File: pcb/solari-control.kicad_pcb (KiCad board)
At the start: 2 copper layers, 80 x 90 mm, 111 parts, among them J1 Conn_01x04, J2 A5081WV-5P, J3 A5081WR-5P, J4 AVR-ISP-6, J5 DIL8, J6 Conn_01x04, Q1 AO3401A, Q10 BC847, Q11 BC857, Q12 BC847, Q2 2N7002, Q3 BC857, Q4 2N7002, Q5 BSS83, Q6 BSS83, Q7 AO3401A, Q8 AO3401A, Q9 BC857, U1 VO0631T, U10 PC817, U11 PC817, U13 ADuM1201AR, U2 L78L05_SOT89, U3 VO0631T, U4 PC817, U5 PC817, U6 VO0631T, U7 ATmega328P-A, U8 VO0631T, U9 VO0631T, Y1 14.7456 MHz

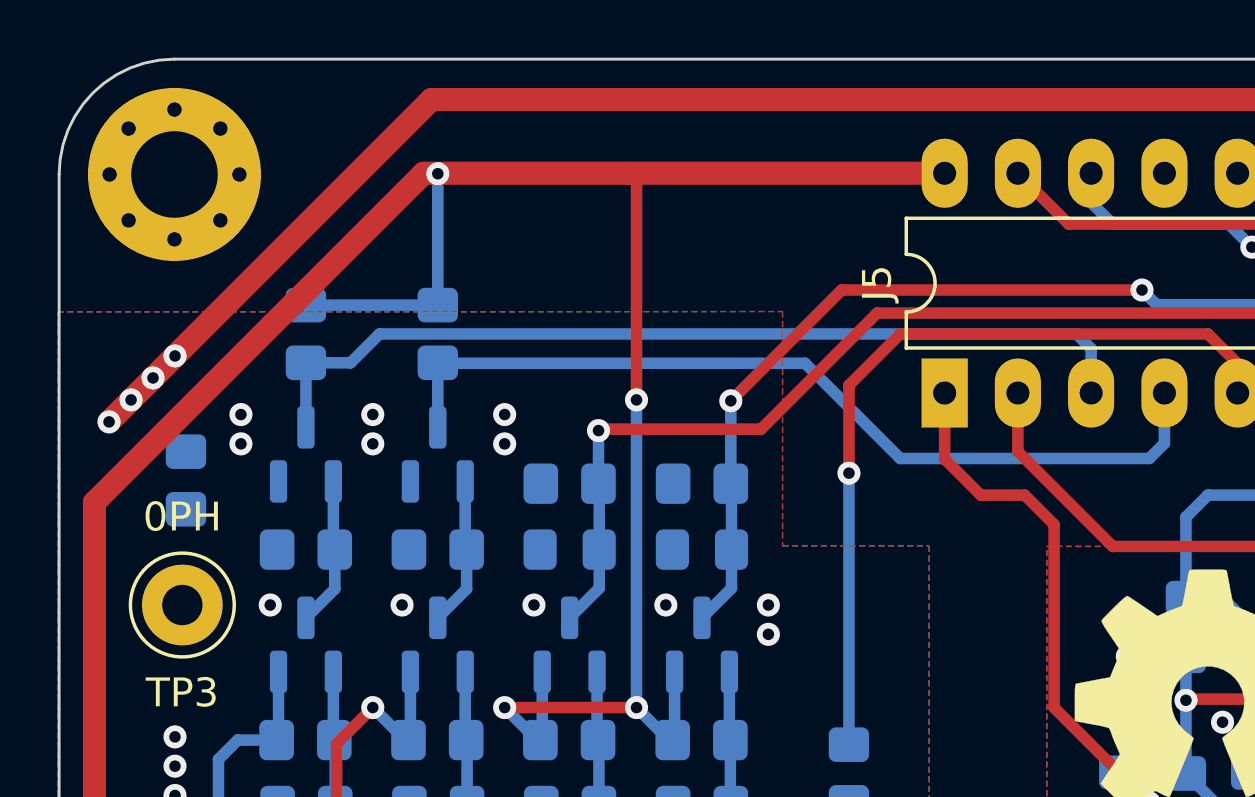
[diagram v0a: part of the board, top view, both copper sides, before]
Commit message: Place new resistor on PCB.
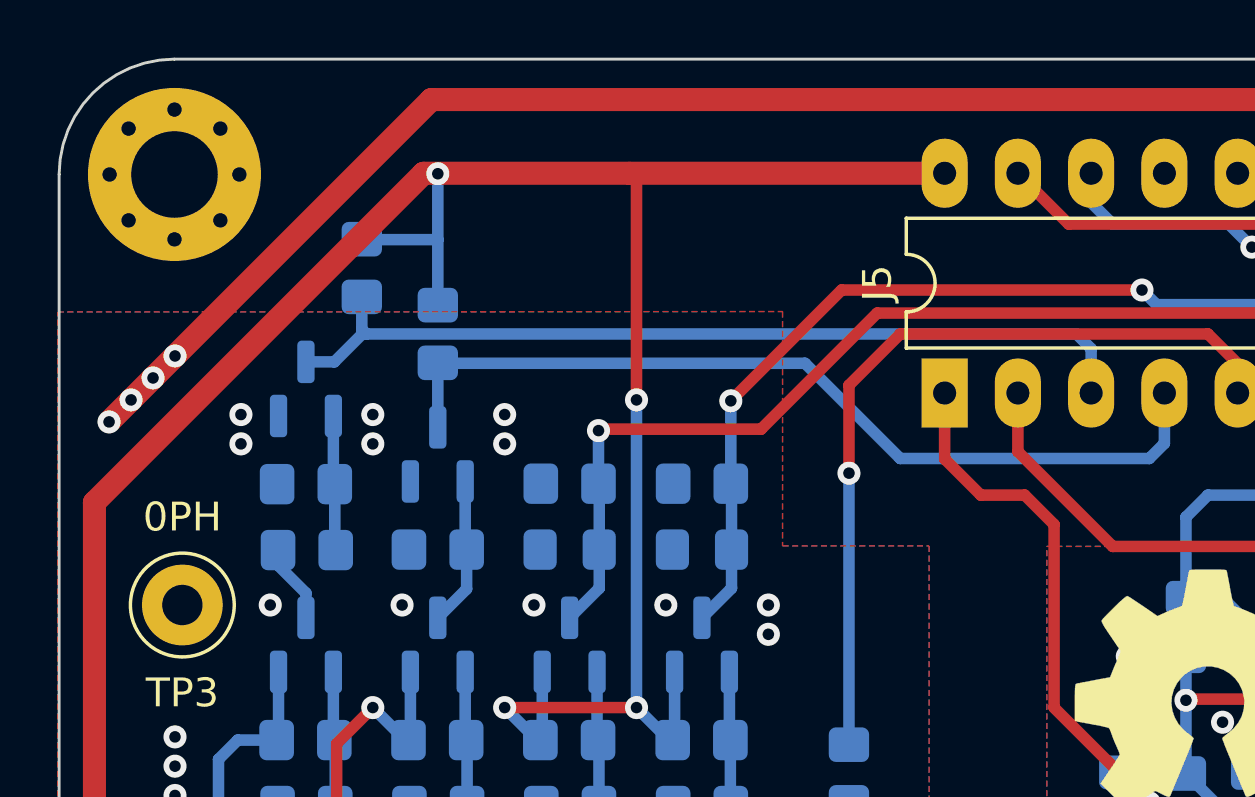
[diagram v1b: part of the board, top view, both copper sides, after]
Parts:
- moved R39 4.84 mm to (148.6, 57.0), turned to 180 degrees
- moved R7 3.00 mm to (150.5, 47.2)
- moved Q4 2.27 mm to (148.6, 51.4)
- moved R12 2.27 mm to (148.6, 54.7)
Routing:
- net Net-(Q3-Pad3): track 0.00 -> 2.75 mm
- net VPH: track 139.3 -> 137.3 mm
- net /CLOCKS: track 31.6 -> 30.7 mm
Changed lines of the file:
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@@
   )
   (footprint "Resistor_SMD:R_0805_2012Metric_Pad1.20x1.40mm_HandSolder" (layer "B.Cu")
-    (at 148.558 57.007)
+    (at 148.558 54.737)
     (descr "Resistor SMD 0805 (2012 Metric), square (rectangular) end terminal, IPC_7351 nominal with elongated pad for handsoldering. (Body size source: IPC-SM-782 page 72, https://www.pcb-3d.com/wordpress/wp-content/uploads/ipc-sm-782a_amendment_1_and_2.pdf), generated with kicad-footprint-generator")
     (tags "resistor handsolder")
@@
   )
   (footprint "Resistor_SMD:R_0805_2012Metric_Pad1.20x1.40mm_HandSolder" (layer "B.Cu")
-    (at 144.399 54.61 -90)
+    (at 148.59 57.023 180)
     (descr "Resistor SMD 0805 (2012 Metric), square (rectangular) end terminal, IPC_7351 nominal with elongated pad for handsoldering. (Body size source: IPC-SM-782 page 72, https://www.pcb-3d.com/wordpress/wp-content/uploads/ipc-sm-782a_amendment_1_and_2.pdf), generated with kicad-footprint-generator")
     (tags "resistor handsolder")
@@
     (property "Sheetname" "")
     (attr smd)
-    (fp_text reference "R39" (at -3.302 -0.508 90) (layer "B.SilkS")
+    (fp_text reference "R39" (at 3.429 0.635) (layer "B.SilkS")
       (effects (font (size 1 1) (thickness 0.15)) (justify mirror))
     )
-    (fp_text value "470R" (at 0 -1.65 90) (layer "B.Fab")
+    (fp_text value "470R" (at 0 -1.65) (layer "B.Fab")
       (effects (font (size 1 1) (thickness 0.15)) (justify mirror))
     )
-    (fp_text user "${REFERENCE}" (at 0 0 90) (layer "B.Fab")
+    (fp_text user "${REFERENCE}" (at 0 0) (layer "B.Fab")
       (effects (font (size 0.5 0.5) (thickness 0.08)) (justify mirror))
     )
@@
     (fp_line (start -1 0.625) (end 1 0.625) (layer "B.Fab") (width 0.1))
     (fp_line (start 1 0.625) (end 1 -0.625) (layer "B.Fab") (width 0.1))
-    (pad "1" smd roundrect (at -1 0 270) (size 1.2 1.4) (layers "B.Cu" "B.Paste" "B.Mask") (roundrect_rratio 0.208333)
+    (pad "1" smd roundrect (at -1 0 180) (size 1.2 1.4) (layers "B.Cu" "B.Paste" "B.Mask") (roundrect_rratio 0.208333)
       (net 109 "Net-(Q4-Pad1)") (pintype "passive"))
-    (pad "2" smd roundrect (at 1 0 270) (size 1.2 1.4) (layers "B.Cu" "B.Paste" "B.Mask") (roundrect_rratio 0.208333)
+    (pad "2" smd roundrect (at 1 0 180) (size 1.2 1.4) (layers "B.Cu" "B.Paste" "B.Mask") (roundrect_rratio 0.208333)
       (net 63 "Net-(Q3-Pad3)") (pintype "passive"))
     (model "${KICAD6_3DMODEL_DIR}/Resistor_SMD.3dshapes/R_0805_2012Metric.wrl"
@@
   )
   (footprint "Package_TO_SOT_SMD:SOT-23" (layer "B.Cu")
-    (at 148.558 53.705 90)
+    (at 148.558 51.435 90)
     (descr "SOT, 3 Pin (https://www.jedec.org/system/files/docs/to-236h.pdf variant AB), generated with kicad-footprint-generator ipc_gullwing_generator.py")
     (tags "SOT TO_SOT_SMD")
@@
   )
   (footprint "Resistor_SMD:R_0805_2012Metric_Pad1.20x1.40mm_HandSolder" (layer "B.Cu")
-    (at 148.558 49.53 90)
+    (at 150.495 47.244 90)
     (descr "Resistor SMD 0805 (2012 Metric), square (rectangular) end terminal, IPC_7351 nominal with elongated pad for handsoldering. (Body size source: IPC-SM-782 page 72, https://www.pcb-3d.com/wordpress/wp-content/uploads/ipc-sm-782a_amendment_1_and_2.pdf), generated with kicad-footprint-generator")
     (tags "resistor handsolder")
@@
     (property "Sheetname" "")
     (attr smd)
-    (fp_text reference "R7" (at 0 1.65 90) (layer "B.SilkS")
+    (fp_text reference "R7" (at 3.048 0 90) (layer "B.SilkS")
       (effects (font (size 1 1) (thickness 0.15)) (justify mirror))
     )
@@
   (via (at 153.13 43.974) (size 0.8) (drill 0.4) (layers "F.Cu" "B.Cu") (net 8))
   (via (at 160.02 51.816) (size 0.8) (drill 0.4) (layers "F.Cu" "B.Cu") (net 8))
-  (segment (start 153.13 48.53) (end 148.558 48.53) (width 0.4) (layer "B.Cu") (net 8))
   (segment (start 161.147 63.611) (end 160.02 62.484) (width 0.4) (layer "B.Cu") (net 8))
+  (segment (start 150.511 46.26) (end 153.13 46.26) (width 0.4) (layer "B.Cu") (net 8))
   (segment (start 161.34 63.545) (end 161.274 63.611) (width 0.4) (layer "B.Cu") (net 8))
+  (segment (start 153.13 48.53) (end 153.13 46.26) (width 0.4) (layer "B.Cu") (net 8))
+  (segment (start 150.495 46.244) (end 150.511 46.26) (width 0.4) (layer "B.Cu") (net 8))
   (segment (start 156.752 63.545) (end 156.686 63.611) (width 0.4) (layer "B.Cu") (net 8))
-  (segment (start 153.13 48.53) (end 153.13 43.974) (width 0.4) (layer "B.Cu") (net 8))
   (segment (start 156.686 63.611) (end 156.575 63.611) (width 0.4) (layer "B.Cu") (net 8))
+  (segment (start 153.13 46.26) (end 153.13 43.974) (width 0.4) (layer "B.Cu") (net 8))
   (segment (start 156.575 63.611) (end 155.448 62.484) (width 0.4) (layer "B.Cu") (net 8))
   (segment (start 156.752 61.2465) (end 156.752 63.545) (width 0.4) (layer "B.Cu") (net 8))
@@
   (segment (start 183.134 58.69) (end 183.134 56.896) (width 0.4) (layer "B.Cu") (net 17))
   (segment (start 184.912 68.58) (end 184.404 68.072) (width 0.4) (layer "B.Cu") (net 17))
-  (segment (start 150.106 50.53) (end 148.558 50.53) (width 0.4) (layer "B.Cu") (net 18))
-  (segment (start 175.783 50.038) (end 175.275 49.53) (width 0.4) (layer "B.Cu") (net 18))
-  (segment (start 175.275 49.53) (end 151.106 49.53) (width 0.4) (layer "B.Cu") (net 18))
-  (segment (start 151.106 49.53) (end 150.106 50.53) (width 0.4) (layer "B.Cu") (net 18))
-  (segment (start 148.558 52.7675) (end 148.558 50.53) (width 0.4) (layer "B.Cu") (net 18))
+  (segment (start 149.5435 50.4975) (end 148.558 50.4975) (width 0.4) (layer "B.Cu") (net 18))
   (segment (start 175.783 51.577) (end 175.783 50.038) (width 0.4) (layer "B.Cu") (net 18))
+  (segment (start 175.275 49.53) (end 150.654 49.53) (width 0.4) (layer "B.Cu") (net 18))
+  (segment (start 175.783 50.038) (end 175.275 49.53) (width 0.4) (layer "B.Cu") (net 18))
+  (segment (start 150.495 49.371) (end 150.654 49.53) (width 0.4) (layer "B.Cu") (net 18))
+  (segment (start 150.511 49.53) (end 149.5435 50.4975) (width 0.4) (layer "B.Cu") (net 18))
+  (segment (start 150.654 49.53) (end 150.511 49.53) (width 0.4) (layer "B.Cu") (net 18))
+  (segment (start 150.495 48.244) (end 150.495 49.371) (width 0.4) (layer "B.Cu") (net 18))
   (segment (start 178.323 53.325) (end 177.8 53.848) (width 0.4) (layer "B.Cu") (net 19))
   (segment (start 177.8 53.848) (end 169.164 53.848) (width 0.4) (layer "B.Cu") (net 19))
@@
   (segment (start 154.13 57.007) (end 154.13 58.3715) (width 0.4) (layer "B.Cu") (net 62))
   (segment (start 154.08 54.6425) (end 154.08 56.957) (width 0.4) (layer "B.Cu") (net 62))
+  (segment (start 148.558 59.3715) (end 148.558 58.515) (width 0.4) (layer "B.Cu") (net 63))
+  (segment (start 148.558 58.515) (end 147.59 57.547) (width 0.4) (layer "B.Cu") (net 63))
+  (segment (start 147.59 57.547) (end 147.59 57.023) (width 0.4) (layer "B.Cu") (net 63))
   (segment (start 163.274 65.881) (end 163.29 65.897) (width 0.4) (layer "B.Cu") (net 64))
   (segment (start 163.24 63.577) (end 163.274 63.611) (width 0.4) (layer "B.Cu") (net 64))
@@
   (segment (start 206.182 54.7855) (end 206.182 57.068) (width 0.4) (layer "B.Cu") (net 108))
   (segment (start 206.182 57.068) (end 206.264 57.15) (width 0.4) (layer "B.Cu") (net 108))
-  (segment (start 149.558 57.007) (end 149.558 58.3715) (width 0.4) (layer "B.Cu") (net 109))
-  (segment (start 149.508 54.6425) (end 149.508 56.957) (width 0.4) (layer "B.Cu") (net 109))
-  (segment (start 149.558 58.3715) (end 148.558 59.3715) (width 0.4) (layer "B.Cu") (net 109))
-  (segment (start 149.508 56.957) (end 149.558 57.007) (width 0.4) (layer "B.Cu") (net 109))
+  (segment (start 149.558 56.991) (end 149.59 57.023) (width 0.4) (layer "B.Cu") (net 109))
+  (segment (start 149.558 54.737) (end 149.558 56.991) (width 0.4) (layer "B.Cu") (net 109))
+  (segment (start 149.508 52.3725) (end 149.508 54.687) (width 0.4) (layer "B.Cu") (net 109))
+  (segment (start 149.508 54.687) (end 149.558 54.737) (width 0.4) (layer "B.Cu") (net 109))
   (zone (net 2) (net_name "0PH") (layers F&B.Cu) (hatch edge 0.508)
     (connect_pads (clearance 0.3))
